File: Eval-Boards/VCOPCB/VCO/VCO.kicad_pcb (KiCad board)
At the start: 2 copper layers, 78.7 x 33 mm, 3 parts

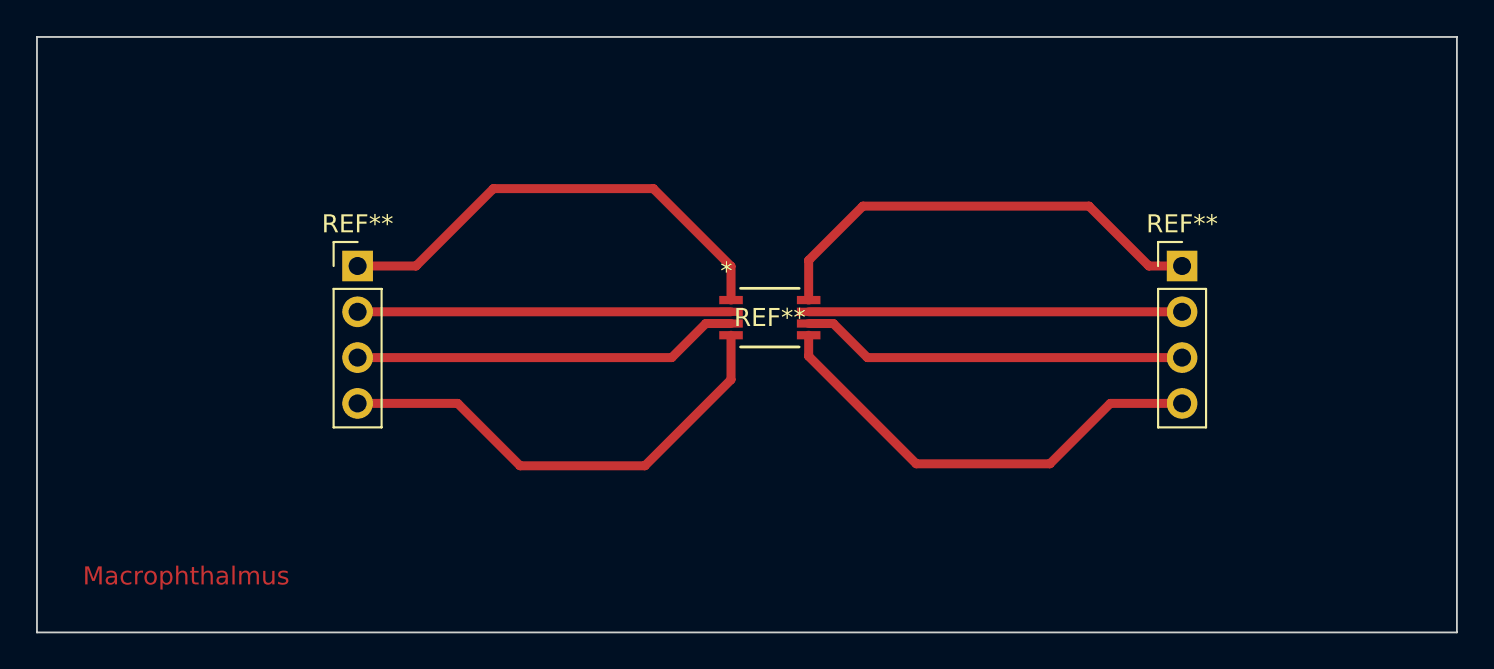
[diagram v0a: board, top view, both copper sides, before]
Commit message: VCO Updated
VCO Fixed
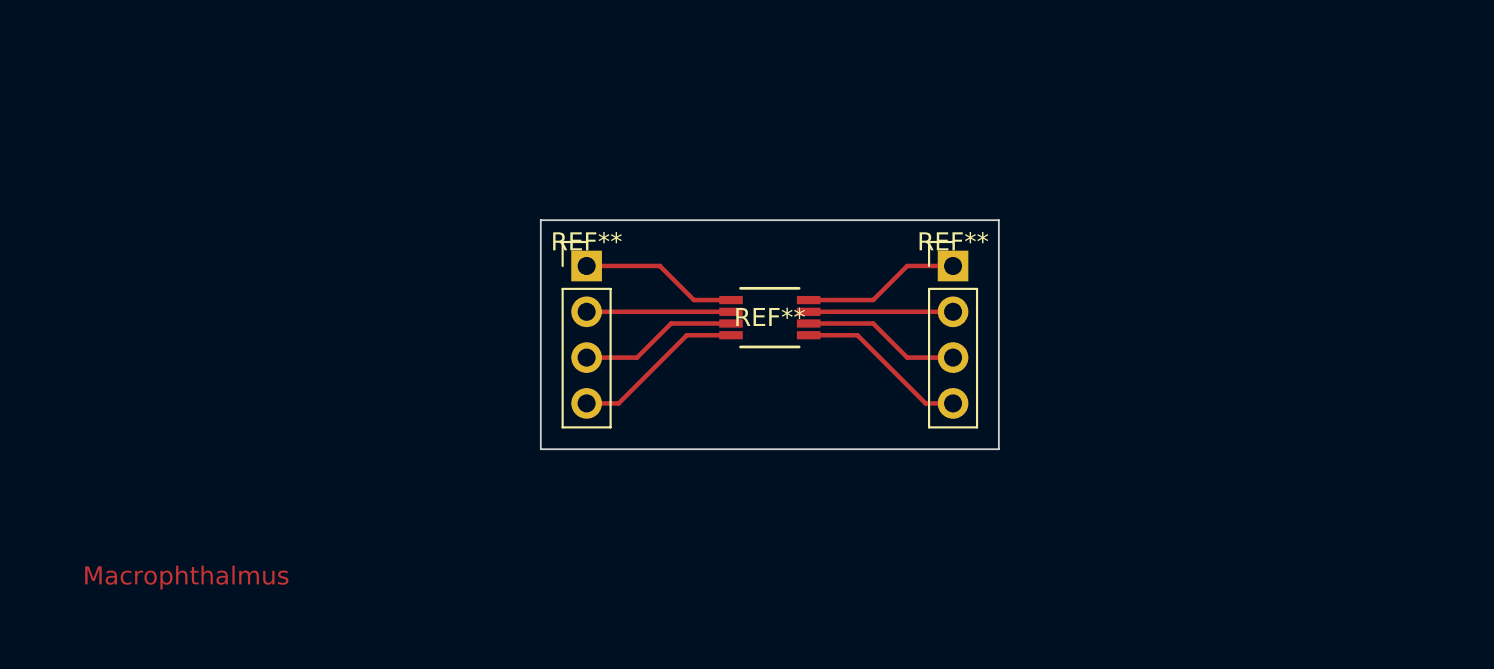
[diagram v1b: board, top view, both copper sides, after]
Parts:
- moved REF** 12.7 mm to (121.9, 91.4)
- moved REF** 12.7 mm to (142.2, 91.4)
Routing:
- net (no net): track 188.4 -> 70.3 mm
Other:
- board size 78.7 x 33 mm -> 25.4 x 12.7 mm
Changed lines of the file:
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@@
   (net 0 "")
   (footprint "Connector_PinHeader_2.54mm:PinHeader_1x04_P2.54mm_Vertical" (layer "F.Cu")
-    (at 154.94 91.44)
+    (at 142.24 91.44)
     (descr "Through hole straight pin header, 1x04, 2.54mm pitch, single row")
     (tags "Through hole pin header THT 1x04 2.54mm single row")
     (attr through_hole)
-    (fp_text reference "REF**" (at 0 -2.33) (layer "F.SilkS")
-        (effects (font (size 1 1) (thickness 0.15)))
-    )
-    (fp_text value "PinHeader_1x04_P2.54mm_Vertical" (at 0 9.95) (layer "F.Fab")
+    (fp_text reference "REF**" (at 0 -1.33) (layer "F.SilkS")
+        (effects (font (size 1 1) (thickness 0.15)))
+    )
+    (fp_text value "PinHeader_1x04_P2.54mm_Vertical" (at 0 9.95) (layer "F.Fab") hide
         (effects (font (size 1 1) (thickness 0.15)))
     )
@@
         (effects (font (size 1 1) (thickness 0.15)))
     )
-    (fp_text value "TSSOP8_3P10X3P10_ONS" (at 0 0 unlocked) (layer "F.Fab")
-        (effects (font (size 1 1) (thickness 0.15)))
-    )
-    (fp_text user "*" (at -2.40665 -2.5752 unlocked) (layer "F.SilkS")
-        (effects (font (size 1 1) (thickness 0.15)))
-    )
-    (fp_text user "*" (at -2.40665 -2.5752) (layer "F.SilkS")
+    (fp_text value "TSSOP8_3P10X3P10_ONS" (at 0 0 unlocked) (layer "F.Fab") hide
         (effects (font (size 1 1) (thickness 0.15)))
     )
@@
   )
   (footprint "Connector_PinHeader_2.54mm:PinHeader_1x04_P2.54mm_Vertical" (layer "F.Cu")
-    (at 109.22 91.44)
+    (at 121.92 91.44)
     (descr "Through hole straight pin header, 1x04, 2.54mm pitch, single row")
     (tags "Through hole pin header THT 1x04 2.54mm single row")
     (attr through_hole)
-    (fp_text reference "REF**" (at 0 -2.33) (layer "F.SilkS")
-        (effects (font (size 1 1) (thickness 0.15)))
-    )
-    (fp_text value "PinHeader_1x04_P2.54mm_Vertical" (at 0 9.95) (layer "F.Fab")
+    (fp_text reference "REF**" (at 0 -1.33) (layer "F.SilkS")
+        (effects (font (size 1 1) (thickness 0.15)))
+    )
+    (fp_text value "PinHeader_1x04_P2.54mm_Vertical" (at 0 9.95) (layer "F.Fab") hide
         (effects (font (size 1 1) (thickness 0.15)))
     )
@@
     )
   )
-  (gr_rect (start 91.44 78.74) (end 170.18 111.76)
+  (gr_rect (start 119.38 88.9) (end 144.78 101.6)
     (stroke (width 0.1) (type default)) (fill none) (layer "Edge.Cuts"))
   (gr_text "Macrophthalmus" (at 93.98 109.22) (layer "F.Cu")
     (effects (font (size 1 1) (thickness 0.15)) (justify left bottom))
   )
-  (segment (start 135.600002 94.630002) (end 137.49 96.52) (width 0.5) (layer "F.Cu") (net 0))
-  (segment (start 134.23265 96.44265) (end 140.2 102.41) (width 0.5) (layer "F.Cu") (net 0))
-  (segment (start 125.15 102.52) (end 118.23 102.52) (width 0.5) (layer "F.Cu") (net 0))
-  (segment (start 134.23265 93.330002) (end 134.23265 91.12735) (width 0.5) (layer "F.Cu") (net 0))
-  (segment (start 129.92735 93.330002) (end 129.92735 91.45735) (width 0.5) (layer "F.Cu") (net 0))
-  (segment (start 116.75 87.15) (end 112.46 91.44) (width 0.5) (layer "F.Cu") (net 0))
-  (segment (start 129.92735 93.98) (end 109.22 93.98) (width 0.5) (layer "F.Cu") (net 0))
-  (segment (start 154.94 93.98) (end 134.23265 93.98) (width 0.5) (layer "F.Cu") (net 0))
-  (segment (start 150.96 99.06) (end 154.94 99.06) (width 0.5) (layer "F.Cu") (net 0))
-  (segment (start 125.62 87.15) (end 116.75 87.15) (width 0.5) (layer "F.Cu") (net 0))
-  (segment (start 118.23 102.52) (end 114.77 99.06) (width 0.5) (layer "F.Cu") (net 0))
-  (segment (start 129.92735 95.28) (end 129.92735 97.74265) (width 0.5) (layer "F.Cu") (net 0))
-  (segment (start 140.2 102.41) (end 147.61 102.41) (width 0.5) (layer "F.Cu") (net 0))
-  (segment (start 128.529998 94.630002) (end 126.64 96.52) (width 0.5) (layer "F.Cu") (net 0))
-  (segment (start 129.92735 91.45735) (end 125.62 87.15) (width 0.5) (layer "F.Cu") (net 0))
-  (segment (start 134.23265 95.28) (end 134.23265 96.44265) (width 0.5) (layer "F.Cu") (net 0))
-  (segment (start 137.24 88.12) (end 149.78 88.12) (width 0.5) (layer "F.Cu") (net 0))
-  (segment (start 129.92735 97.74265) (end 125.15 102.52) (width 0.5) (layer "F.Cu") (net 0))
-  (segment (start 149.78 88.12) (end 153.1 91.44) (width 0.5) (layer "F.Cu") (net 0))
-  (segment (start 137.49 96.52) (end 154.94 96.52) (width 0.5) (layer "F.Cu") (net 0))
-  (segment (start 112.46 91.44) (end 109.22 91.44) (width 0.5) (layer "F.Cu") (net 0))
-  (segment (start 153.1 91.44) (end 154.94 91.44) (width 0.5) (layer "F.Cu") (net 0))
-  (segment (start 147.61 102.41) (end 150.96 99.06) (width 0.5) (layer "F.Cu") (net 0))
-  (segment (start 126.64 96.52) (end 109.22 96.52) (width 0.5) (layer "F.Cu") (net 0))
-  (segment (start 134.23265 91.12735) (end 137.24 88.12) (width 0.5) (layer "F.Cu") (net 0))
-  (segment (start 129.92735 94.630002) (end 128.529998 94.630002) (width 0.5) (layer "F.Cu") (net 0))
-  (segment (start 134.23265 94.630002) (end 135.600002 94.630002) (width 0.5) (layer "F.Cu") (net 0))
-  (segment (start 114.77 99.06) (end 109.22 99.06) (width 0.5) (layer "F.Cu") (net 0))
+  (segment (start 124.714 96.52) (end 126.603998 94.630002) (width 0.25) (layer "F.Cu") (net 0))
+  (segment (start 140.716 99.06) (end 142.24 99.06) (width 0.25) (layer "F.Cu") (net 0))
+  (segment (start 121.92 93.98) (end 129.92735 93.98) (width 0.25) (layer "F.Cu") (net 0))
+  (segment (start 125.984 91.44) (end 121.92 91.44) (width 0.25) (layer "F.Cu") (net 0))
+  (segment (start 139.7 91.44) (end 142.24 91.44) (width 0.25) (layer "F.Cu") (net 0))
+  (segment (start 121.92 99.06) (end 123.698 99.06) (width 0.25) (layer "F.Cu") (net 0))
+  (segment (start 134.23265 94.630002) (end 137.810002 94.630002) (width 0.25) (layer "F.Cu") (net 0))
+  (segment (start 137.810002 94.630002) (end 139.7 96.52) (width 0.25) (layer "F.Cu") (net 0))
+  (segment (start 134.23265 93.98) (end 142.24 93.98) (width 0.25) (layer "F.Cu") (net 0))
+  (segment (start 139.7 96.52) (end 142.24 96.52) (width 0.25) (layer "F.Cu") (net 0))
+  (segment (start 134.23265 95.28) (end 136.936 95.28) (width 0.25) (layer "F.Cu") (net 0))
+  (segment (start 121.92 96.52) (end 124.714 96.52) (width 0.25) (layer "F.Cu") (net 0))
+  (segment (start 134.23265 93.330002) (end 137.809998 93.330002) (width 0.25) (layer "F.Cu") (net 0))
+  (segment (start 126.603998 94.630002) (end 129.92735 94.630002) (width 0.25) (layer "F.Cu") (net 0))
+  (segment (start 137.809998 93.330002) (end 139.7 91.44) (width 0.25) (layer "F.Cu") (net 0))
+  (segment (start 136.936 95.28) (end 140.716 99.06) (width 0.25) (layer "F.Cu") (net 0))
+  (segment (start 127.478 95.28) (end 129.92735 95.28) (width 0.25) (layer "F.Cu") (net 0))
+  (segment (start 123.698 99.06) (end 127.478 95.28) (width 0.25) (layer "F.Cu") (net 0))
+  (segment (start 127.874002 93.330002) (end 125.984 91.44) (width 0.25) (layer "F.Cu") (net 0))
+  (segment (start 129.92735 93.330002) (end 127.874002 93.330002) (width 0.25) (layer "F.Cu") (net 0))
 )
